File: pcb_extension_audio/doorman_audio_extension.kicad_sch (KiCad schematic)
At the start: 52 parts, among them J1 Output, J2 GPIO, J3 Input, J4 Extension Board Connector, U2 ES8311

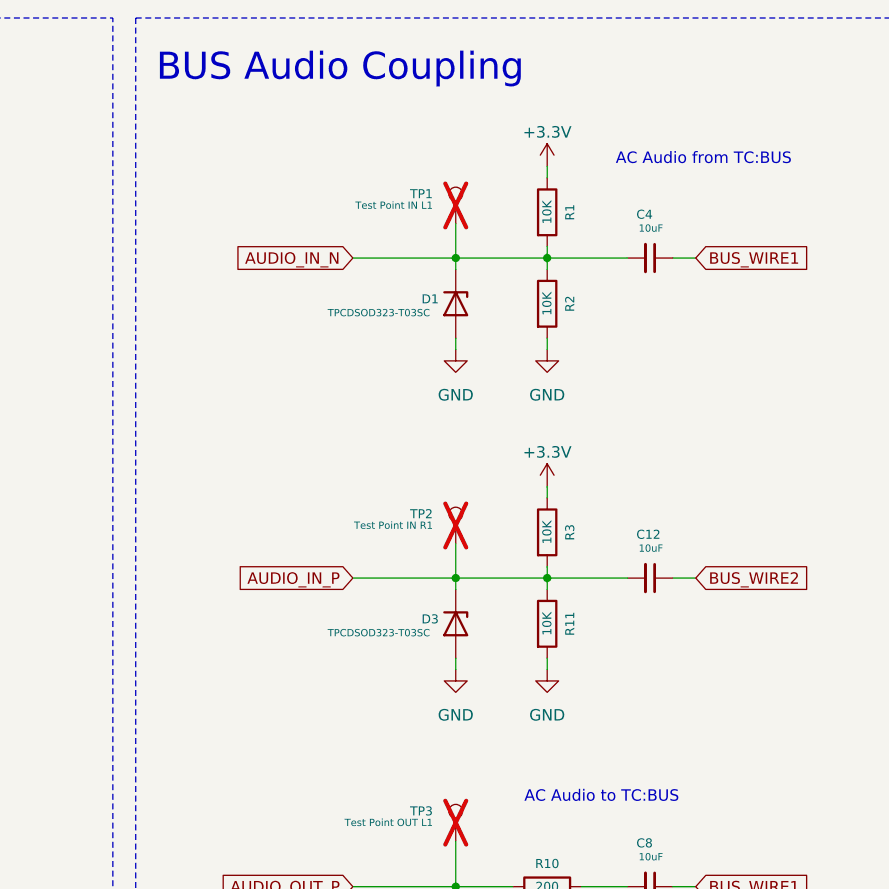
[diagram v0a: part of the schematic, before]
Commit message: WIP
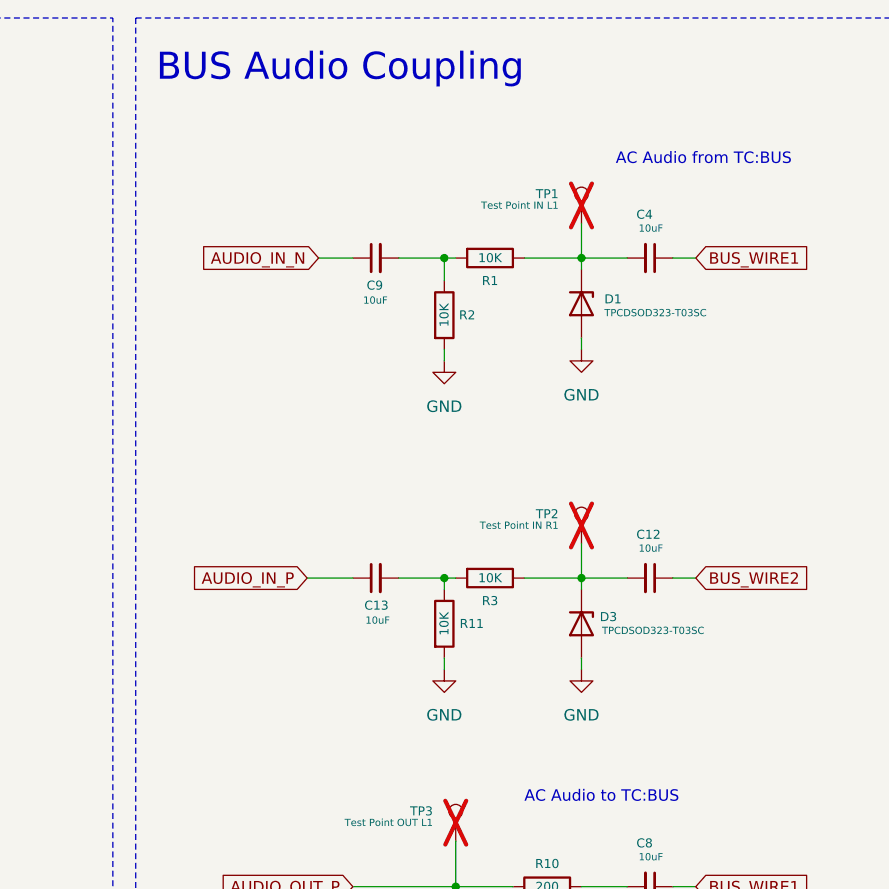
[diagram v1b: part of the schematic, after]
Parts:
- added C13, C9: 10uF, Capacitor_SMD:C_0402_1005Metric, symbol Device:C_Small
- C11, C17, C19, C2, C21: LCSC C19702 -> C2959727; MPN CL10A106KP8NNNC -> GRM188Z71A106KA73D
- C3, C5, C6, C7: LCSC (none) -> C29936; MPN (none) -> CL10B105KA8NNNC
- R10, R6: LCSC C25361 -> C18002; MPN 1206W4J0201T5E -> 1206W4F2000T5E
- U2: LCSC (none) -> C962342; MPN (none) -> ES8311
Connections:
- net +3.3V: no longer R1.1, R3.1
- net AUDIO_IN_N: now also C9.1; no longer C4.2, D1.1 (K), R1.2, R2.1, TP1.1
- net AUDIO_IN_P: now also C13.1; no longer C12.2, D3.1 (K), R11.1, R3.2, TP2.1
- new net: C4.2, D1.1 (K), R1.1, TP1.1
- new net: C13.2, R11.1, R3.2
- new net: C9.2, R1.2, R2.1
- new net: C12.2, D3.1 (K), R3.1, TP2.1
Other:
- moved on the sheet: D1, D3, R1, R11, R2, R3, TP1, TP2
